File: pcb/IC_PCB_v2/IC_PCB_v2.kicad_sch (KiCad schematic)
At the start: 17 parts, among them IC1 MAX30102EFD+, IC2 MAX30205MTA+, J1 52207-0460, U1 AZ1084-1.8

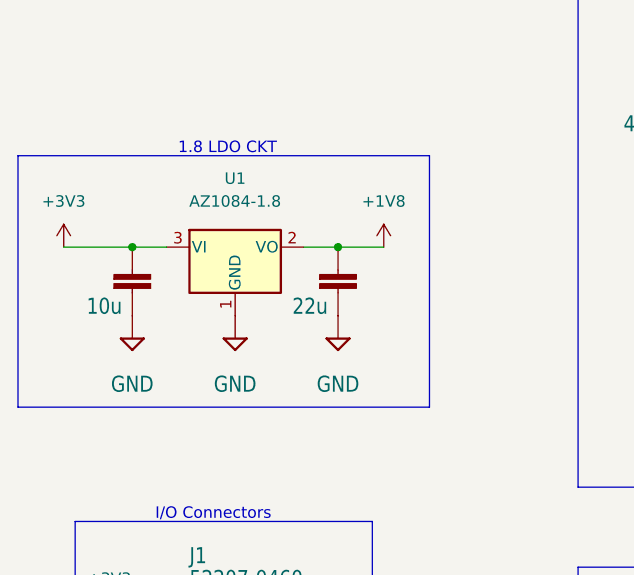
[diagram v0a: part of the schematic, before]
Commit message: uploaded code and stuff
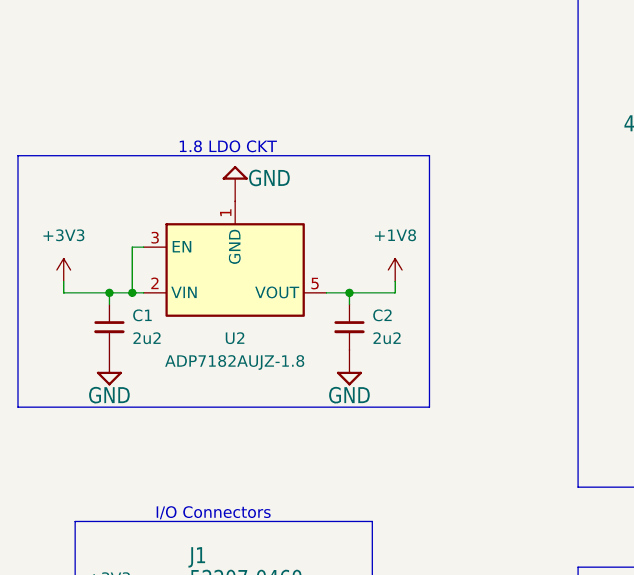
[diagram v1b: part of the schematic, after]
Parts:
- removed C1: 10u, Capacitor_SMD:C_1206_3216Metric, symbol IC_PCB-eagle-import:C2,5-3
- removed C2: 22u, Capacitor_SMD:C_1206_3216Metric, symbol IC_PCB-eagle-import:C2,5-3
- removed U1: AZ1084-1.8, Package_TO_SOT_SMD:TO-252-3_TabPin2, symbol Regulator_Linear:AZ1084-1.8
- added C1, C2: 2u2, Capacitor_SMD:C_0603_1608Metric, symbol Device:C_Small
- added U2: ADP7182AUJZ-1.8, Package_TO_SOT_SMD:TSOT-23-5, symbol Regulator_Linear:ADP7182AUJZ-1.8
- C3, C7: footprint Capacitor_SMD:C_0201_0603Metric_Pad0.64x0.40mm_HandSolder -> Capacitor_SMD:C_0603_1608Metric
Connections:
- net +1V8: now also C2.1, U2.5 (VOUT)
- net +3V3: now also C1.1, U2.2 (VIN), U2.3 (EN)
- net GND: now also C1.2, C2.2, U2.1 (GND)
